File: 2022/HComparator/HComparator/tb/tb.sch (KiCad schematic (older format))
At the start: 3 parts

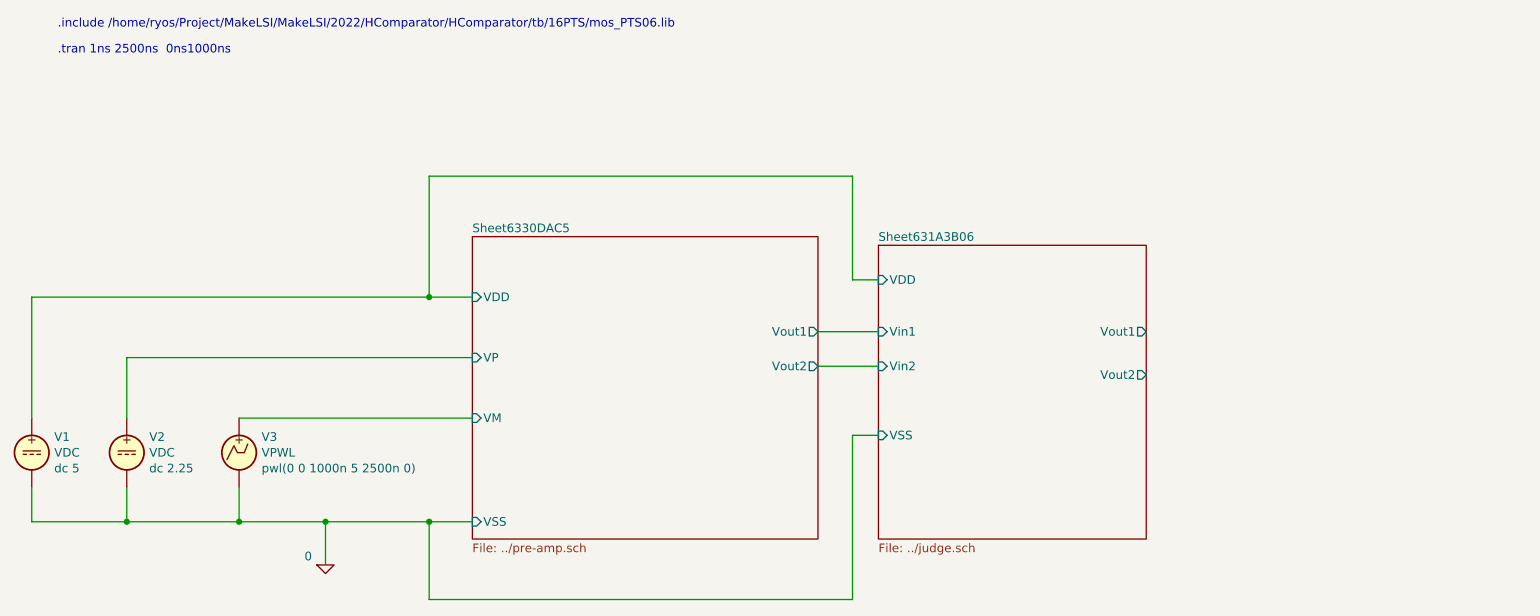
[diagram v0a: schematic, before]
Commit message: とりあえず TB は通った。
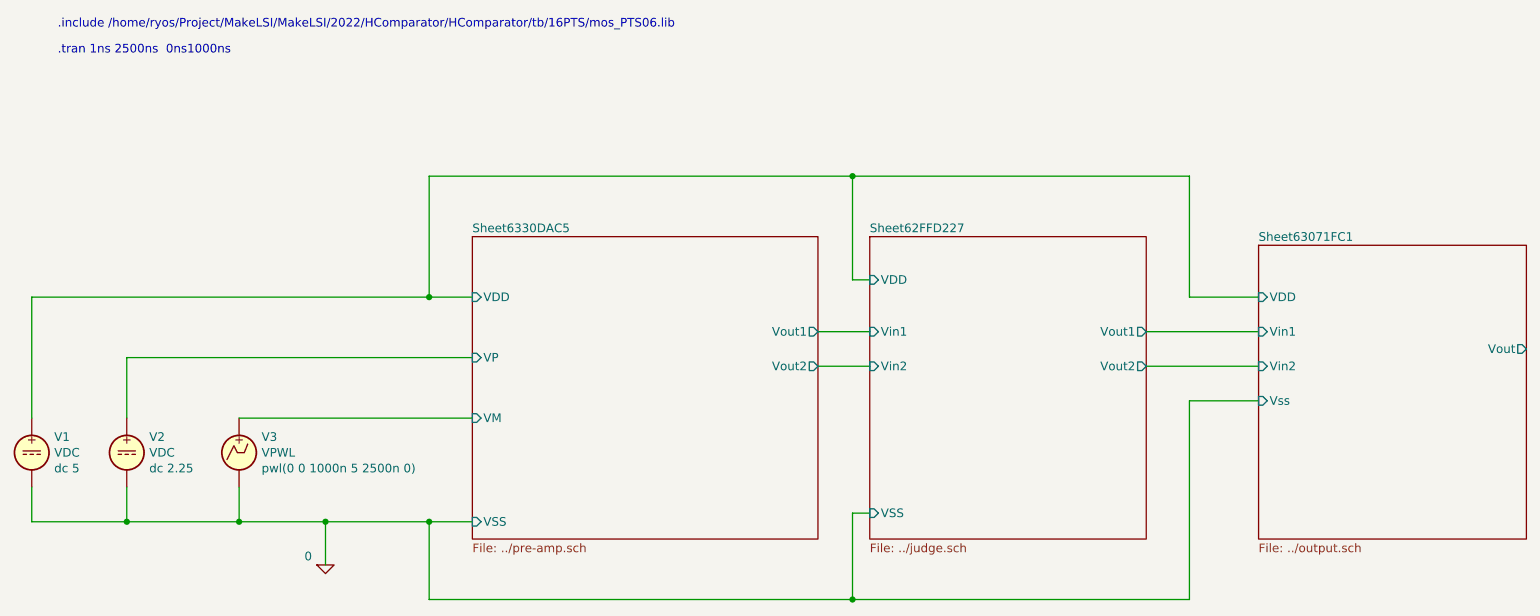
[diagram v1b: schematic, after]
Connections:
- net Sheet631A3B06/VDD renamed Sheet62FFD227/VDD
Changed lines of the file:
@@
 $Descr A4 11693 8268
 encoding utf-8
-Sheet 1 3
+Sheet 1 4
 Title ""
 Date ""
@@
 Wire Wire Line
 	4550 3350 4300 3350
-$Sheet
-S 6900 3050 1550 1700
-U 631A3B07
-F0 "Sheet631A3B06" 50
-F1 "../judge.sch" 50
-F2 "VDD" I L 6900 3250 50
-F3 "Vin1" I L 6900 3550 50
-F4 "Vin2" I L 6900 3750 50
-F5 "VSS" I L 6900 4150 50
-F6 "Vout1" O R 8450 3550 50
-F7 "Vout2" O R 8450 3800 50
-$EndSheet
-Wire Wire Line
-	6550 3550 6900 3550
-Wire Wire Line
-	6550 3750 6900 3750
 Wire Wire Line
 	4300 3350 4300 2650
 Wire Wire Line
-	4300 2650 6750 2650
-Wire Wire Line
 	6750 2650 6750 3250
-Wire Wire Line
-	6750 3250 6900 3250
 Connection ~ 4300 3350
 Wire Wire Line
@@
 	4300 5100 6750 5100
 Wire Wire Line
-	6750 5100 6750 4150
-Wire Wire Line
-	6750 4150 6900 4150
+	6750 5100 6750 4600
 Connection ~ 4300 4650
 Wire Wire Line
 	4300 4650 3700 4650
+Wire Wire Line
+	4300 2650 6750 2650
+Wire Wire Line
+	6750 5100 8700 5100
+Connection ~ 6750 5100
+Connection ~ 6750 2650
+Wire Wire Line
+	6750 2650 8700 2650
+$Sheet
+S 6850 3000 1600 1750
+U 62FFD228
+F0 "Sheet62FFD227" 50
+F1 "../judge.sch" 50
+F2 "VDD" I L 6850 3250 50
+F3 "Vin1" I L 6850 3550 50
+F4 "Vin2" I L 6850 3750 50
+F5 "VSS" I L 6850 4600 50
+F6 "Vout1" O R 8450 3550 50
+F7 "Vout2" O R 8450 3750 50
+$EndSheet
+Wire Wire Line
+	6850 4600 6750 4600
+Wire Wire Line
+	6550 3550 6850 3550
+Wire Wire Line
+	6550 3750 6850 3750
+Wire Wire Line
+	6750 3250 6850 3250
+Wire Wire Line
+	8700 2650 8700 3350
+Wire Wire Line
+	8700 3950 8700 5100
+$Sheet
+S 9100 3050 1550 1700
+U 63071FC2
+F0 "Sheet63071FC1" 50
+F1 "../output.sch" 50
+F2 "VDD" I L 9100 3350 50
+F3 "Vin1" I L 9100 3550 50
+F4 "Vin2" I L 9100 3750 50
+F5 "Vss" I L 9100 3950 50
+F6 "Vout" O R 10650 3650 50
+$EndSheet
+Wire Wire Line
+	8700 3350 9100 3350
+Wire Wire Line
+	8450 3550 9100 3550
+Wire Wire Line
+	8450 3750 9100 3750
+Wire Wire Line
+	8700 3950 9100 3950
 $EndSCHEMATC
